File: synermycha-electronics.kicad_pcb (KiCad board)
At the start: 4 copper layers, 50 x 75 mm, 168 parts, among them J12 Conn_01x05, J13 Conn_01x05, J14 Conn_01x05, J15 Conn_01x05, J16 Conn_01x05, J17 CK-JS102011SAQN, J2 Conn_01x02, J3 Conn_01x02, J4 USB_C_Receptacle_USB2.0, J6 A1250WV-S-4P, J7 Conn_01x04, J8 Conn_01x04, Q1 SSM6J507NU, Q2 SSM6J507NU, Q3 SSM6J507NU, Q4 BC847, Q5 BC856, SW1 DTSM32N, SW2 DTSM32N, SW3 DTSM32N, SW4 DTSM32N, U1 LM1117LDX, U12 MPU-9250, U13 STM32F446RETx, U14 STM14_SW, U2 LDFM33PVR, U3 RN4871U-V_RM118, U4 DRV8835, U5 MCP73213, U6 ETA3000, U7 STUSB4500QTR, Y1 16Mhz, 18pF

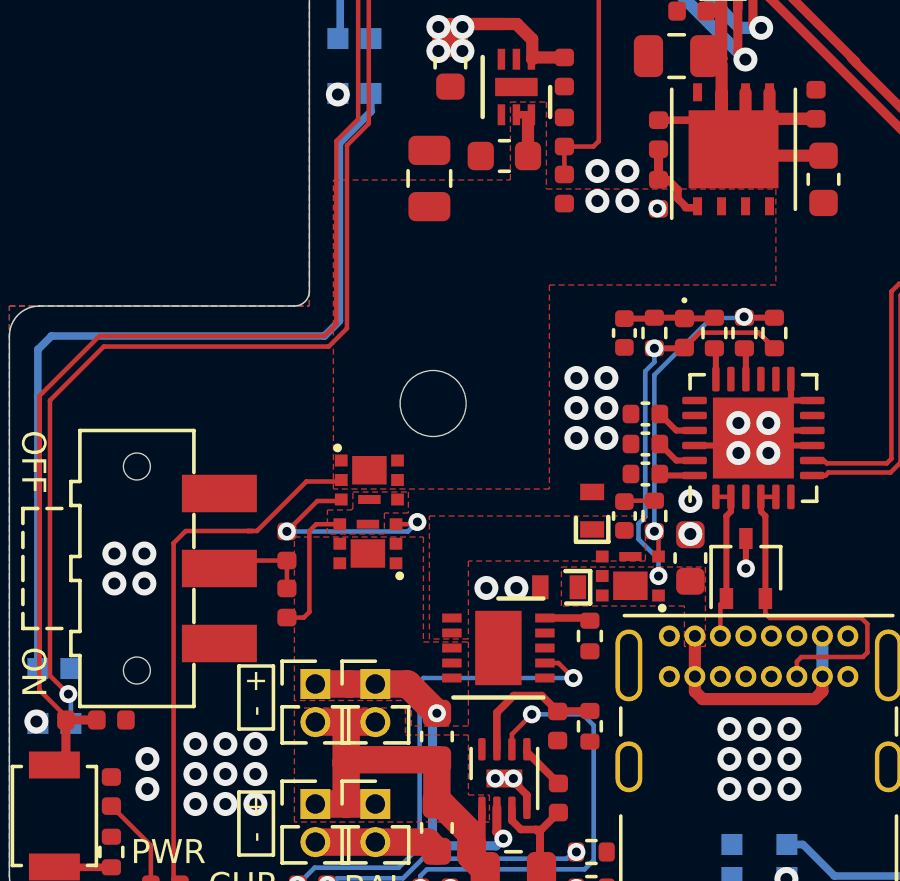
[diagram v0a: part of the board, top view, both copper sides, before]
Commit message: Kosmetyka
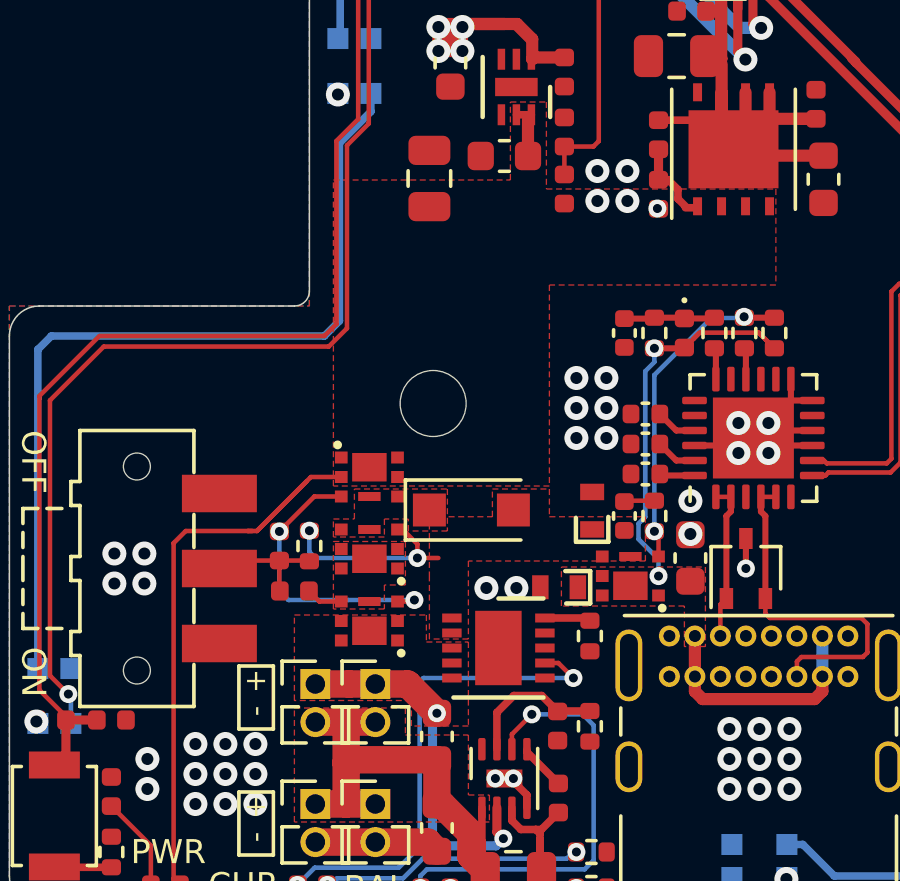
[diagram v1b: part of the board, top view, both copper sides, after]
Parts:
- added D30: 30V,2A, Diode_SMD:D_SOD-123F, F.Cu at (27.4, 184.8)
- added Q6: SSM6J507NU, footprints:UDFN6B, F.Cu at (24.0, 186.1)
- added R34: 100K, Resistor_SMD:R_0402_1005Metric, F.Cu at (22.0, 186.0)
- C26: value 0.1uF -> 10uF
- moved Q1 2.58 mm to (24.0, 188.5)
- moved R51 0.47 mm to (21.5, 187.5), turned to 0 degrees
- moved R52 0.25 mm to (21.0, 186.0)
- moved Q3 0.10 mm to (24.0, 183.7)
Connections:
- Q3 pad 4: Net-(Q1-Pad4) -> Net-(D30-Pad1)
- Q3 pad S: Net-(Q1-Pad4) -> Net-(D30-Pad1)
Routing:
- net /Power Section/VDRIVE: track 0.00 -> 6.42 mm, vias 0 -> 2
- net Net-(Q1-Pad4): track 4.63 -> 1.22 mm
- net /Power Section/VCC: track 19.8 -> 22.2 mm
- net Net-(Q1-Pad3): track 7.43 -> 9.74 mm
- net Net-(J17-Pad2): track 3.29 -> 4.30 mm
- added copper zone on F.Cu, net Net-(D30-Pad1)
